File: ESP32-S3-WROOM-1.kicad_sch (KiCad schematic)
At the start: 24 parts, among them J11 Conn_01x08, J13 Conn_02x09_Top_Bottom, J14 Conn_01x09, J15 Conn_02x09_Top_Bottom, J4 B4B-ZRLFSN, J6 Conn_01x09, J7 Conn_02x20_Counter_Clockwise, J8 Conn_01x08, J9 Conn_01x08, SW4 SW_Push, U8 ESP32-S3-WROOM-1-N8R2

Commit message: JLCniceness
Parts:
- J4: value B4B-ZRLFSN -> JST-XH; footprint JST-ZR-4Pin:CONN_B4B-ZRLFSN_JST -> Connector_JST:JST_XH_B4B-XH-AM_1x04_P2.50mm_Vertical
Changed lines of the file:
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@@
 			)
 		)
-		(property "Value" "B4B-ZRLFSN"
+		(property "Value" "JST-XH"
 			(at 283.21 159.766 0)
 			(effects
@@
 			)
 		)
-		(property "Footprint" "JST-ZR-4Pin:CONN_B4B-ZRLFSN_JST"
+		(property "Footprint" "Connector_JST:JST_XH_B4B-XH-AM_1x04_P2.50mm_Vertical"
 			(at 269.748 154.686 0)
 			(effects
@@
 			)
 		)
-		(property "Datasheet" "B4B-ZRLFSN"
+		(property "Datasheet" ""
 			(at 269.748 154.686 0)
 			(effects
@@
 			(at 269.748 154.686 0)
 			(effects
-				(font
-					(size 1.27 1.27)
-				)
-				(hide yes)
-			)
-		)
-		(property "JLCPCB Position Offset" ""
-			(at 269.748 154.686 0)
-			(effects

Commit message: JLC fixes
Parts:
- J4: footprint Connector_JST:JST_XH_B4B-XH-AM_1x04_P2.50mm_Vertical -> Connector_JST:JST_XH_B4B-XH-A_1x04_P2.50mm_Vertical
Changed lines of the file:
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@@
 			)
 		)
-		(property "Footprint" "Connector_JST:JST_XH_B4B-XH-AM_1x04_P2.50mm_Vertical"
+		(property "Footprint" "Connector_JST:JST_XH_B4B-XH-A_1x04_P2.50mm_Vertical"
 			(at 269.748 154.686 0)
 			(effects
@@
 			(effects
 				(font
+					(size 1.27 1.27)
+				)
+				(hide yes)
+			)
+		)
+		(property "LCSC Part # " ""
+			(at 0 309.372 0)
+			(effects
+				(font

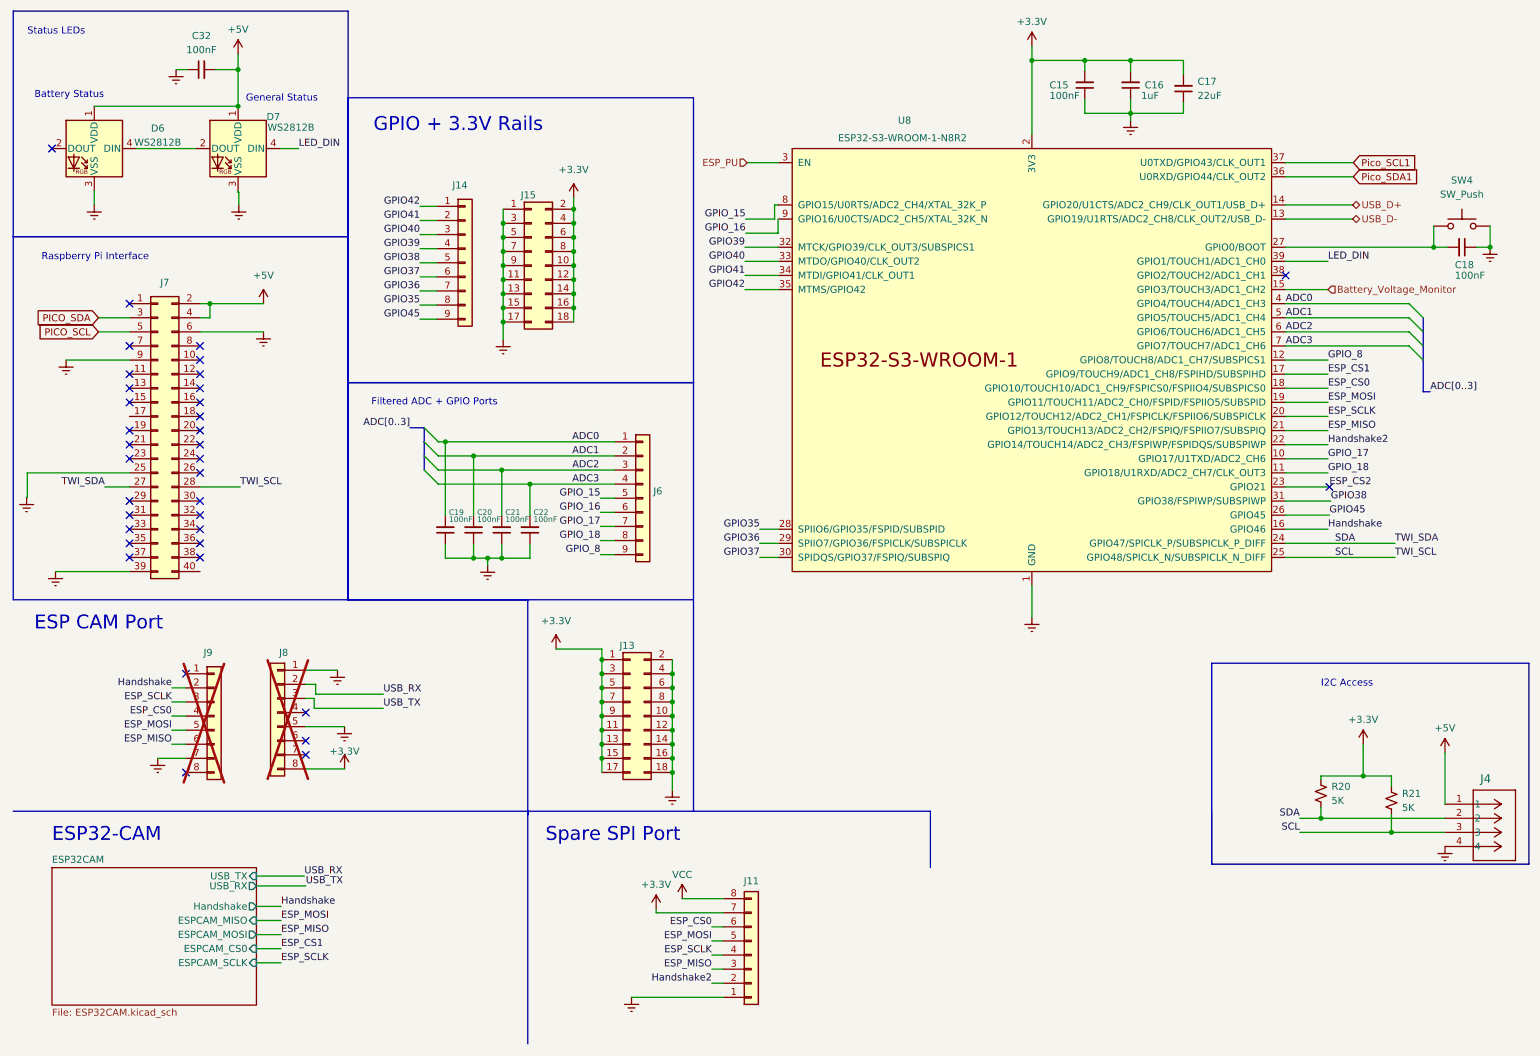
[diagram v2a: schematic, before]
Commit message: Rev 2 PCB
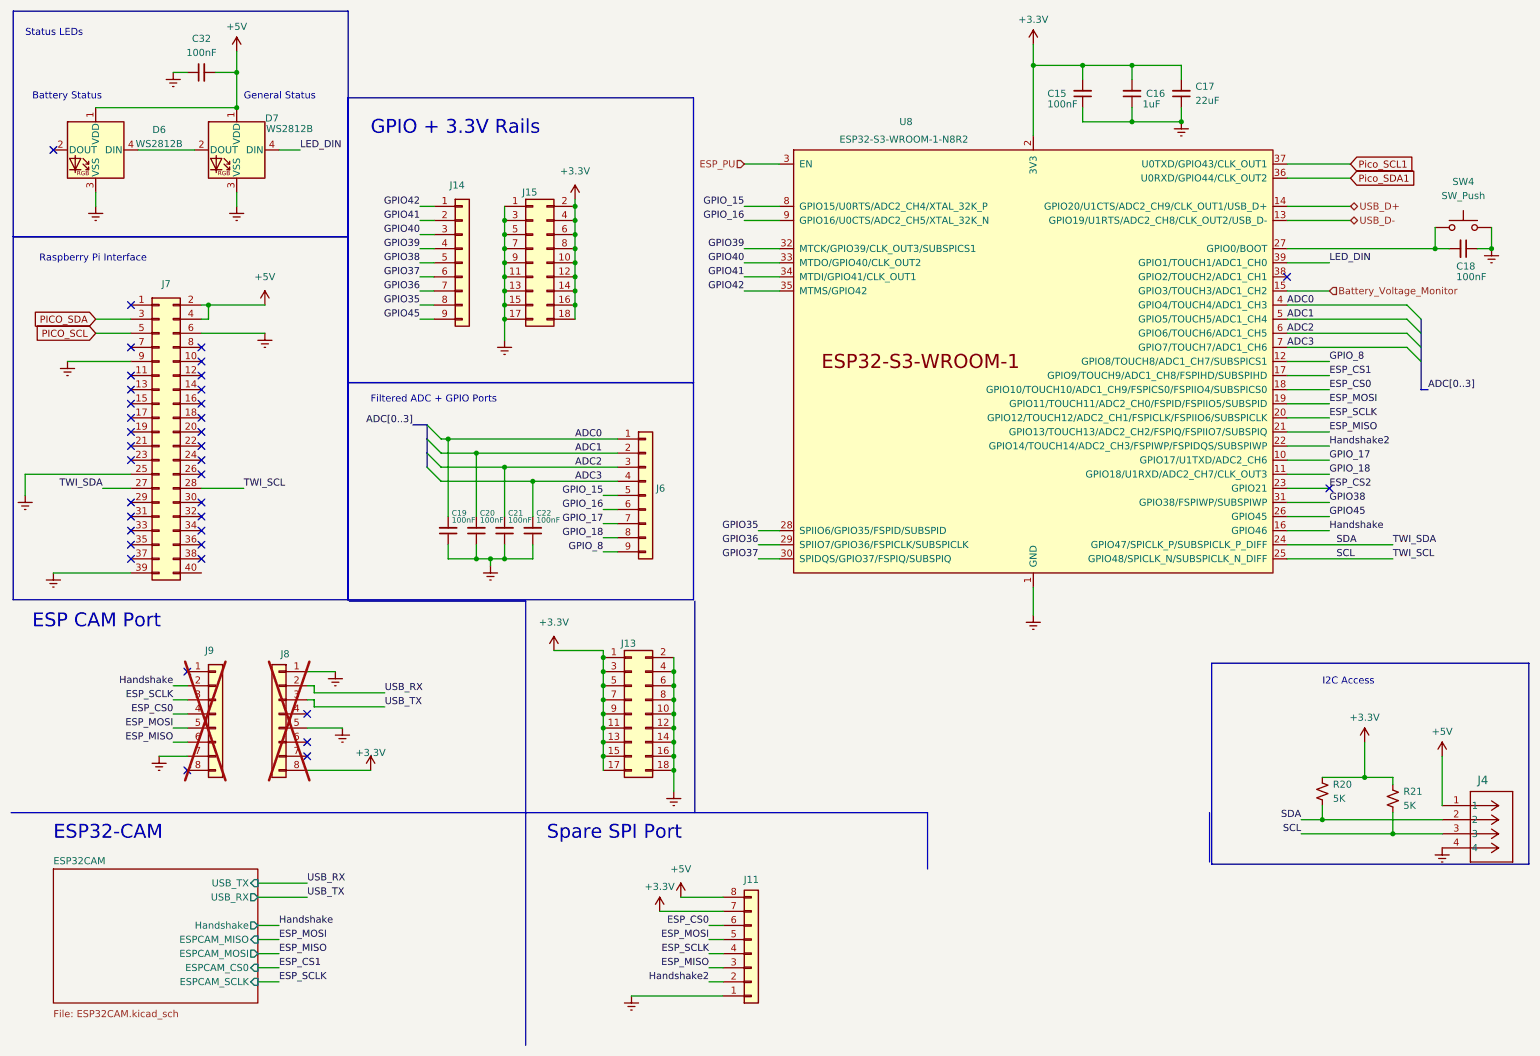
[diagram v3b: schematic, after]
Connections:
- net VCC is gone; now on net +5V: J11.8 (Pin_8)
- no-connect marks 36 -> 37
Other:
- moved on the sheet: C15, C16, C17, C19, C20, C21, C22, C32, J14, J15, J4, J6
